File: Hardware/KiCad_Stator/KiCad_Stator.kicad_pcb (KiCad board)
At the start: 2 copper layers, 29.5 x 29.5 mm, 0 parts

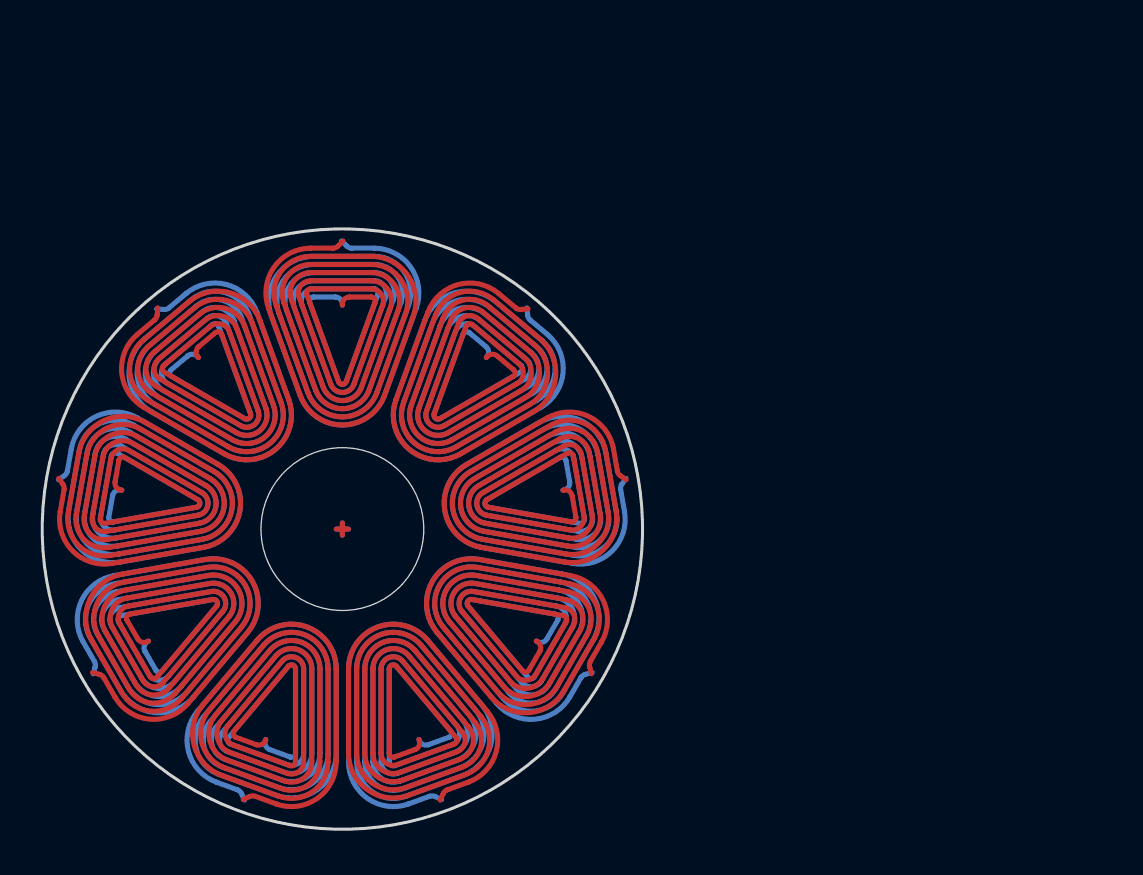
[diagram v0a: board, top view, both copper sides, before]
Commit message: feat:prototype v0.1
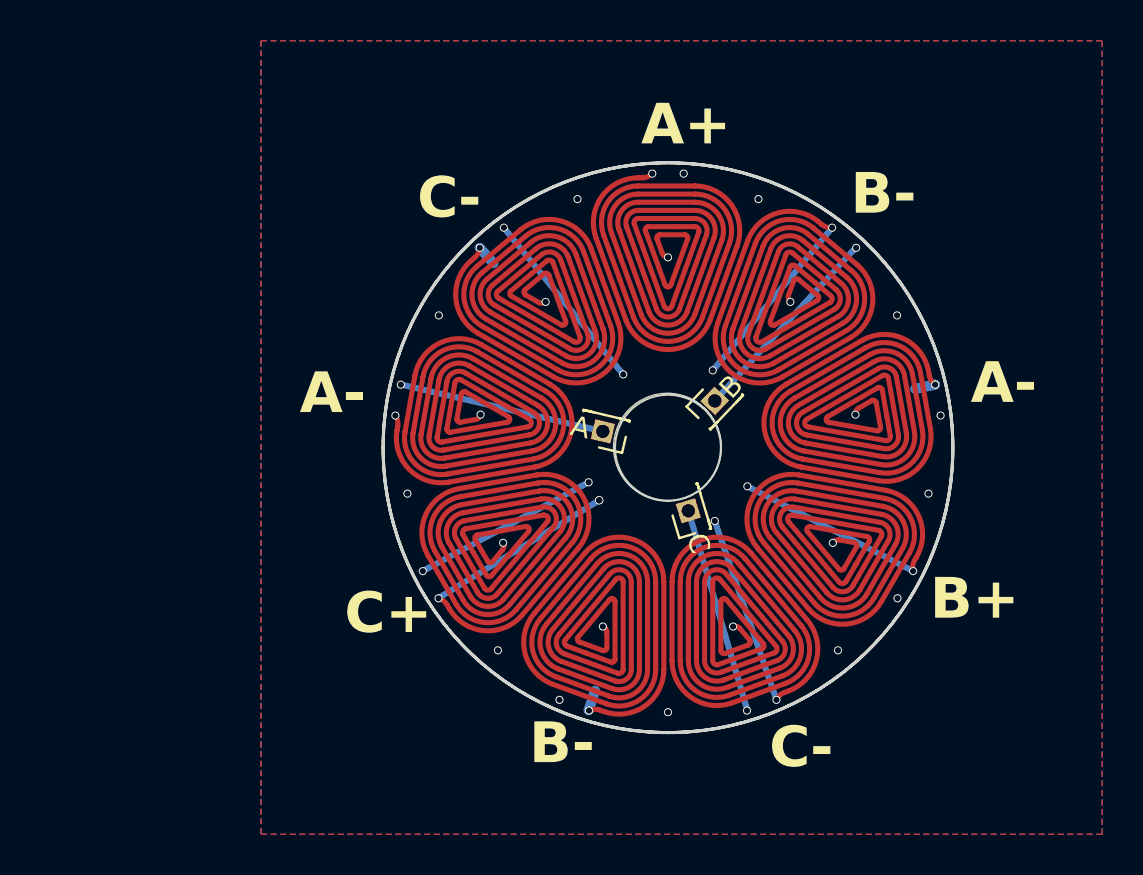
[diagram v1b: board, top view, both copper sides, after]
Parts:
- added A1: B, Connector_PinHeader_1.27mm:PinHeader_1x01_P1.27mm_Vertical, F.Cu at (160.3, 71.7)
- added B1: A, Connector_PinHeader_1.27mm:PinHeader_1x01_P1.27mm_Vertical, F.Cu at (154.8, 73.2)
- added C1: C, Connector_PinHeader_1.27mm:PinHeader_1x01_P1.27mm_Vertical, F.Cu at (159.0, 77.1)
- added H1: MountingHole, MountingHole:MountingHole_5.3mm_M5, F.Cu at (158.0, 74.0)
- added NT1: NetTie_2, NetTie:NetTie-2_SMD_Pad0.5mm, B.Cu at (154.3, 86.4)
- added NT2: NetTie_2, NetTie:NetTie-2_SMD_Pad0.5mm, B.Cu at (170.6, 71.0)
- added NT3: NetTie_2, NetTie:NetTie-2_SMD_Pad0.5mm, B.Cu at (149.1, 64.6)
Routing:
- net /B: track 0.00 -> 4.69 mm, vias 0 -> 9
- net /A: track 0.00 -> 2.77 mm, vias 0 -> 11
- net GND: vias 0 -> 9
- net /C: vias 0 -> 14
- added copper zone on B.Cu, net GND
- added copper zone on F.Cu, net GND
- added copper zone on In1.Cu, net GND
- added copper zone on In2.Cu, net GND
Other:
- board size 29.5 x 29.5 mm -> 28 x 28 mm
- copper layers 2 -> 4
- board text added: "+ rot in - grün in"
- board text added: "A+"
- board text added: "A-"
- board text added: "B+"
- board text added: "B-"
- board text added: "C+"
- board text added: "C-"
